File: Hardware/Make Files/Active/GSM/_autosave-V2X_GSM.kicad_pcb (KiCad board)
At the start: 2 copper layers, 85 x 56 mm, 44 parts, among them P1 SIM_SKT, P14 CUR_SEN, P2 SMA, P26 CONN_02X10, P3 SMA, Q12 IRF9335, U13 XRP6124, U24 TLV70012DCK, U3 MMQA5V6T3G, U4 SIM5320

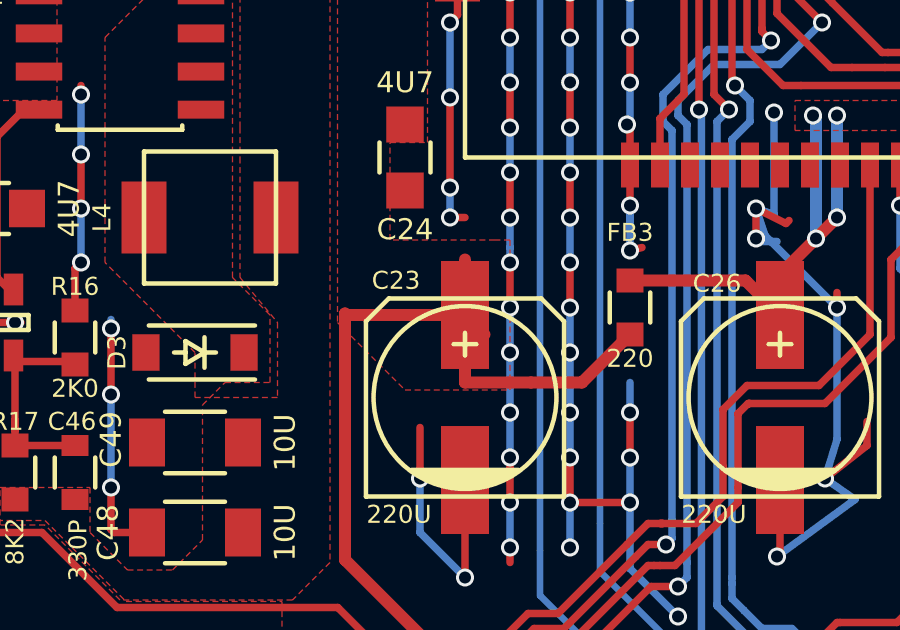
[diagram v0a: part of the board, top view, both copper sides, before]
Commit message: Project Shares and Next rev cleanup
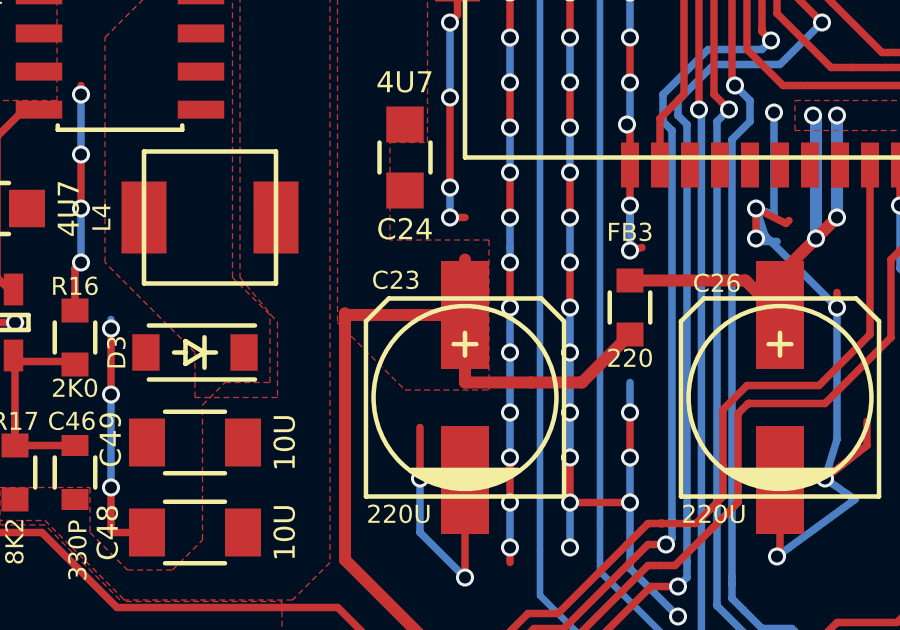
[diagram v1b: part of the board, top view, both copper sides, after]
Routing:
- net 4V1_B: track 60.4 -> 59.5 mm
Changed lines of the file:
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@@
     (thickness 1.6)
     (drawings 18)
-    (tracks 1504)
+    (tracks 1503)
     (zones 0)
     (modules 44)
@@
       (drillshape 0)
       (scaleselection 1)
-      (outputdirectory C:/Users/jbanks2/Documents/Projects/rvi_v2x_board/Hardware/Gerbers/Active/))
+      (outputdirectory "C:/Users/jbanks2/Documents/Projects/rvi_v2x_board/Hardware/Project Shares/V1.2/"))
   )
   (net 0 "")
@@
   (segment (start 131.72 135.5) (end 132.2 135.5) (width 0.4) (layer B.Cu) (net 17))
   (segment (start 134 121.8) (end 134 121.24918) (width 0.4) (layer F.Cu) (net 17))
-  (segment (start 134 121.24918) (end 134.65082 121.9) (width 0.4) (layer F.Cu) (net 17))
   (segment (start 134 121.24918) (end 134 119.4) (width 0.4) (layer F.Cu) (net 17))
   (segment (start 151.1 129.5) (end 148.3 132.3) (width 0.25) (layer F.Cu) (net 19))
@@
       (pts
         (xy 115.5 106.25) (xy 125.25 106.25) (xy 126.25 106.25) (xy 129.75 109.75) (xy 129.75 121.5)
-        (xy 132 123.75) (xy 135.5 123.75) (xy 135.5 118.75) (xy 135 118.75) (xy 131.5 118.75)
+        (xy 132 123.75) (xy 134.8 123.75) (xy 134.8 118.85) (xy 134.8 118.75) (xy 131.5 118.75)
         (xy 131.5 115.5) (xy 132.75 115.5) (xy 132.75 110) (xy 134.45 110) (xy 134.45 108)
         (xy 130.75 108) (xy 127.75 105) (xy 127.25 104.5) (xy 115.5 104.5) (xy 115.5 104.75)
